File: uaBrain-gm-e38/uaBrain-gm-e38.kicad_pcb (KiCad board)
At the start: 4 copper layers, 130 x 138 mm, 3 parts, among them J1 Molex_313874018 80-pin grey, J2 Molex_313872014 73-pin black, M1 hw-uaBrain

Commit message: Upd SCH
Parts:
- added C1: 100n, hellen-one-common:C0603, F.Cu at (409.8, 70.6)
- added C10: 100n, hellen-one-common:C0603, F.Cu at (413.2, 72.6)
- added C11: 160p, hellen-one-common:C0603, F.Cu at (413.2, 74.5)
- added C12: 160p, hellen-one-common:C0603, F.Cu at (413.2, 76.5)
- added C13: 160p, hellen-one-common:C0603, F.Cu at (413.2, 78.4)
- added C14: 160p, hellen-one-common:C0603, F.Cu at (413.2, 80.4)
- added C15: 160p, hellen-one-common:C0603, F.Cu at (413.2, 82.3)
- added C16: 160p, hellen-one-common:C0603, F.Cu at (413.2, 84.3)
- added C17: 160p, hellen-one-common:C0603, F.Cu at (416.6, 70.6)
- added C18: 160p, hellen-one-common:C0603, F.Cu at (416.6, 72.6)
- added C19: 1u, hellen-one-common:C0603, F.Cu at (416.6, 74.5)
- added C2: 100n, hellen-one-common:C0603, F.Cu at (409.8, 72.6)
- added C20: 1u, hellen-one-common:C0603, F.Cu at (416.6, 76.5)
- added C21: 1u, hellen-one-common:C0603, F.Cu at (416.6, 78.4)
- added C22: 10n, Capacitor_SMD:C_0603_1608Metric, F.Cu at (410.7, 36.0)
- added C23: 10n, Capacitor_SMD:C_0603_1608Metric, F.Cu at (410.7, 38.5)
- added C24: 10n, Capacitor_SMD:C_0603_1608Metric, F.Cu at (410.7, 41.0)
- added C25: 10n, Capacitor_SMD:C_0603_1608Metric, F.Cu at (410.7, 43.6)
- added C26: 10n, Capacitor_SMD:C_0603_1608Metric, F.Cu at (410.7, 46.1)
- added C3: 100n, hellen-one-common:C0603, F.Cu at (409.8, 74.5)
- added C4: 100n, hellen-one-common:C0603, F.Cu at (409.8, 76.5)
- added C5: 100n, hellen-one-common:C0603, F.Cu at (409.8, 78.4)
- added C6: 100n, hellen-one-common:C0603, F.Cu at (409.8, 80.4)
- added C7: 100n, hellen-one-common:C0603, F.Cu at (409.8, 82.3)
- added C8: 100n, hellen-one-common:C0603, F.Cu at (409.8, 84.3)
- added C9: 100n, hellen-one-common:C0603, F.Cu at (413.2, 70.6)
- added D1: SRV05-4-P-T7, Package_TO_SOT_SMD:SOT-23-6, F.Cu at (397.4, 89.6)
- added D2: SRV05-4-P-T7, Package_TO_SOT_SMD:SOT-23-6, F.Cu at (397.4, 94.3)
- added D3: B5819W, hellen-one-common:SOD-123, F.Cu at (406.1, 36.3)
- added D4: B5819W, hellen-one-common:SOD-123, F.Cu at (406.1, 39.5)
- added D5: B5819W, hellen-one-common:SOD-123, F.Cu at (406.1, 42.6)
- added D6: B5819W, hellen-one-common:SOD-123, F.Cu at (406.1, 45.7)
- added D7: B5819W, hellen-one-common:SOD-123, F.Cu at (406.1, 48.8)
- added J3: 5569-06A2, Connector_Molex:Molex_Mini-Fit_Jr_5569-06A2_2x03_P4.20mm_Horizontal, B.Cu at (159.7, 142.7)
- added J4: 5569-06A2, Connector_Molex:Molex_Mini-Fit_Jr_5569-06A2_2x03_P4.20mm_Horizontal, B.Cu at (91.7, 142.7)
- added J5: 5569-04A2, Connector_Molex:Molex_Mini-Fit_Jr_5569-04A2_2x02_P4.20mm_Horizontal, B.Cu at (108.8, 142.7)
- added J6: 5569-16A2, Connector_Molex:Molex_Mini-Fit_Jr_5569-16A2_2x08_P4.20mm_Horizontal, B.Cu at (121.3, 142.7)
- added R1: 100, Resistor_SMD:R_2512_6332Metric_Pad1.40x3.35mm_HandSolder, F.Cu at (345.5, 60.5)
- added R10: DNP, hellen-one-common:R0603, F.Cu at (396.5, 82.4)
- added R11: 470k, hellen-one-common:R0603, F.Cu at (396.5, 84.3)
- added R12: DNP, hellen-one-common:R0603, F.Cu at (396.5, 86.3)
- added R13: 470k, hellen-one-common:R0603, F.Cu at (399.8, 70.7)
- added R14: DNP, hellen-one-common:R0603, F.Cu at (399.8, 72.6)
- added R15: 470k, hellen-one-common:R0603, F.Cu at (399.8, 74.6)
- added R16: DNP, hellen-one-common:R0603, F.Cu at (399.8, 76.5)
- added R17: 470k, hellen-one-common:R0603, F.Cu at (399.8, 78.5)
- added R18: DNP, hellen-one-common:R0603, F.Cu at (399.8, 80.4)
- added R19: 470k, hellen-one-common:R0603, F.Cu at (399.8, 82.4)
- added R2: 100, Resistor_SMD:R_2512_6332Metric_Pad1.40x3.35mm_HandSolder, F.Cu at (345.5, 65.4)
- added R20: 10k, hellen-one-common:R0603, F.Cu at (399.8, 84.3)
- added R21: 10k, hellen-one-common:R0603, F.Cu at (399.8, 86.3)
- added R22: 10k, hellen-one-common:R0603, F.Cu at (403.1, 70.7)
- added R23: 10k, hellen-one-common:R0603, F.Cu at (403.1, 72.6)
- added R24: 10k, hellen-one-common:R0603, F.Cu at (403.1, 74.6)
- added R25: 10k, hellen-one-common:R0603, F.Cu at (403.1, 76.5)
- added R26: 10k, hellen-one-common:R0603, F.Cu at (403.1, 78.5)
- added R27: 10k, hellen-one-common:R0603, F.Cu at (403.1, 80.4)
- added R28: 10k, hellen-one-common:R0603, F.Cu at (403.1, 82.4)
- added R29: 10k, hellen-one-common:R0603, F.Cu at (403.1, 84.3)
- added R3: 100, Resistor_SMD:R_2512_6332Metric_Pad1.40x3.35mm_HandSolder, F.Cu at (345.5, 70.3)
- added R30: 10k, hellen-one-common:R0603, F.Cu at (403.1, 86.3)
- added R31: 10k, hellen-one-common:R0603, F.Cu at (406.4, 70.7)
- added R32: 10k, hellen-one-common:R0603, F.Cu at (406.4, 72.6)
- added R33: 10k, hellen-one-common:R0603, F.Cu at (406.4, 74.6)
- added R34: 10k, hellen-one-common:R0603, F.Cu at (406.4, 76.5)
- added R35: 10k, hellen-one-common:R0603, F.Cu at (406.4, 78.5)
- added R36: 4.7k, hellen-one-common:R0603, F.Cu at (404.9, 51.4)
- added R37: 4.7k, hellen-one-common:R0603, F.Cu at (404.9, 53.3)
- added R38: 4.7k, hellen-one-common:R0603, F.Cu at (404.9, 55.2)
- added R39: 4.7k, hellen-one-common:R0603, F.Cu at (404.9, 57.2)
- added R4: DNP, hellen-one-common:R0603, F.Cu at (396.5, 70.7)
- added R40: 4.7k, hellen-one-common:R0603, F.Cu at (404.9, 59.1)
- added R41: 120, hellen-one-common:R0603, F.Cu at (408.2, 51.4)
- added R42: 120, hellen-one-common:R0603, F.Cu at (408.2, 53.3)
- added R43: 120, hellen-one-common:R0603, F.Cu at (408.2, 55.2)
- added R44: 120, hellen-one-common:R0603, F.Cu at (408.2, 57.2)
- added R45: 120, hellen-one-common:R0603, F.Cu at (408.2, 59.1)
- added R46: 10k, hellen-one-common:R0603, F.Cu at (411.5, 51.4)
- added R47: 10k, hellen-one-common:R0603, F.Cu at (411.5, 53.3)
- added R48: 10k, hellen-one-common:R0603, F.Cu at (411.5, 55.2)
- added R49: 10k, hellen-one-common:R0603, F.Cu at (411.5, 57.2)
- added R5: 470k, hellen-one-common:R0603, F.Cu at (396.5, 72.6)
- added R50: 10k, hellen-one-common:R0603, F.Cu at (411.5, 59.1)
- added R51: 4.7k, hellen-one-common:R0603, F.Cu at (354.3, 82.4)
- added R52: 4.7k, hellen-one-common:R0603, F.Cu at (354.3, 84.3)
- added R53: 4.7k, hellen-one-common:R0603, F.Cu at (354.3, 86.2)
- added R54: 4.7k, hellen-one-common:R0603, F.Cu at (354.3, 88.2)
- added R55: 4.7k, hellen-one-common:R0603, F.Cu at (357.6, 82.4)
- added R56: 4.7k, hellen-one-common:R0603, F.Cu at (357.6, 84.3)
- added R57: 4.7k, hellen-one-common:R0603, F.Cu at (357.6, 86.2)
- added R58: 4.7k, hellen-one-common:R0603, F.Cu at (357.6, 88.2)
- added R59: 4.7k, hellen-one-common:R0603, F.Cu at (360.9, 82.4)
- added R6: DNP, hellen-one-common:R0603, F.Cu at (396.5, 74.6)
- added R60: 4.7k, hellen-one-common:R0603, F.Cu at (360.9, 84.3)
- added R61: 4.7k, hellen-one-common:R0603, F.Cu at (360.9, 86.2)
- added R62: 4.7k, hellen-one-common:R0603, F.Cu at (360.9, 88.2)
- added R63: 4.7k, hellen-one-common:R0603, F.Cu at (351.1, 92.1)
- added R64: 4.7k, hellen-one-common:R0603, F.Cu at (351.1, 94.1)
- added R65: 4.7k, hellen-one-common:R0603, F.Cu at (351.1, 96.0)
- added R66: 4.7k, hellen-one-common:R0603, F.Cu at (351.1, 98.0)
- added R67: 4.7k, hellen-one-common:R0603, F.Cu at (354.4, 92.1)
- added R68: 4.7k, hellen-one-common:R0603, F.Cu at (354.4, 94.1)
- added R69: 4.7k, hellen-one-common:R0603, F.Cu at (354.4, 96.0)
- added R7: 470k, hellen-one-common:R0603, F.Cu at (396.5, 76.5)
- added R70: 4.7k, hellen-one-common:R0603, F.Cu at (354.4, 98.0)
- added R71: 4.7k, hellen-one-common:R0603, F.Cu at (357.7, 92.1)
- added R72: 4.7k, hellen-one-common:R0603, F.Cu at (357.7, 94.1)
- added R73: 4.7k, hellen-one-common:R0603, F.Cu at (357.7, 96.0)
- added R74: 4.7k, hellen-one-common:R0603, F.Cu at (357.7, 98.0)
- added R8: DNP, hellen-one-common:R0603, F.Cu at (396.5, 78.5)
- added R9: 470k, hellen-one-common:R0603, F.Cu at (396.5, 80.4)
- added U1: PCA9685PW, Package_SO:TSSOP-28_4.4x9.7mm_P0.65mm, F.Cu at (345.4, 78.5)
- added U10: VNLD5160TR-E, Package_SO:SOIC-8_3.9x4.9mm_P1.27mm, F.Cu at (371.0, 39.0)
- added U11: VNLD5160TR-E, Package_SO:SOIC-8_3.9x4.9mm_P1.27mm, F.Cu at (371.0, 45.6)
- added U12: VNLD5160TR-E, Package_SO:SOIC-8_3.9x4.9mm_P1.27mm, F.Cu at (371.0, 52.2)
- added U13: VNLD5160TR-E, Package_SO:SOIC-8_3.9x4.9mm_P1.27mm, F.Cu at (345.2, 94.5)
- added U14: VNLD5160TR-E, Package_SO:SOIC-8_3.9x4.9mm_P1.27mm, F.Cu at (345.2, 101.1)
- added U15: VNLD5160TR-E, Package_SO:SOIC-8_3.9x4.9mm_P1.27mm, F.Cu at (345.2, 107.7)
- added U2: MCP6004, Package_SO:TSSOP-14_4.4x5mm_P0.65mm, F.Cu at (412.4, 88.7)
- added U3: MCP6004, Package_SO:TSSOP-14_4.4x5mm_P0.65mm, F.Cu at (412.4, 95.4)
- added U4: ADS7128, Package_DFN_QFN:WQFN-16-1EP_3x3mm_P0.5mm_EP1.68x1.68mm_ThermalVias, F.Cu at (403.0, 89.9)
- added U5: BSP762TXUMA1, Package_SO:SOIC-8_3.9x4.9mm_P1.27mm, F.Cu at (399.1, 38.1)
- added U6: BSP762TXUMA1, Package_SO:SOIC-8_3.9x4.9mm_P1.27mm, F.Cu at (399.1, 44.7)
- added U7: BSP762TXUMA1, Package_SO:SOIC-8_3.9x4.9mm_P1.27mm, F.Cu at (399.1, 51.3)
- added U8: BSP762TXUMA1, Package_SO:SOIC-8_3.9x4.9mm_P1.27mm, F.Cu at (399.1, 57.9)
- added U9: BSP762TXUMA1, Package_SO:SOIC-8_3.9x4.9mm_P1.27mm, F.Cu at (399.1, 64.5)
- J1: renamed from J2; value Molex_313872014 73-pin black -> Molex_313872014_singleside
- J2: renamed from J1; value Molex_313874018 80-pin grey -> Molex_313874018_singleside
- M1: footprint kicad6-libraries:hw-uaBrain -> kicad6-libraries:hw-uaBrain-PinHeader
- moved M1 50.6 mm to (64.2, 143.6)
- moved J1 46.7 mm to (79.3, 75.9)
- moved J2 44.6 mm to (169.2, 75.8)
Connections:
- net CAN_H renamed /uaBrain-gm-e38/CAN_H
- net CAN_L renamed /uaBrain-gm-e38/CAN_L
- net IN_CAM renamed /uaBrain-gm-e38/IN_CAM
- net IN_CLT renamed /uaBrain-gm-e38/IN_CLT
- net IN_CLUTCH_SWITCH renamed /uaBrain-gm-e38/IN_CLUTCH_SWITCH
- net IN_CRANK renamed /uaBrain-gm-e38/IN_CRANK
- net IN_DIN1 renamed /uaBrain-gm-e38/IN_DIN1
- net IN_IAT renamed /uaBrain-gm-e38/IN_IAT
- net IN_KNOCK1 renamed /uaBrain-gm-e38/IN_KNOCK1
- net IN_KNOCK2 renamed /uaBrain-gm-e38/IN_KNOCK2
- net IN_MAF renamed /uaBrain-gm-e38/IN_MAF
- net IN_MAP renamed /uaBrain-gm-e38/IN_MAP
- net IN_OIL_PRESSURE renamed /uaBrain-gm-e38/IN_OIL_PRESSURE
- net IN_PPS1 renamed /uaBrain-gm-e38/IN_PPS1
- net IN_PPS2 renamed /uaBrain-gm-e38/IN_PPS2
- net IN_P/N_SWITCH renamed /uaBrain-gm-e38/IN_P/N_SWITCH
- net IN_STOP_SWITCH renamed /uaBrain-gm-e38/IN_STOP_SWITCH
- net IN_TPS1 renamed /uaBrain-gm-e38/IN_TPS1
- net IN_TPS2 renamed /uaBrain-gm-e38/IN_TPS2
- net OUT_AC_RELAY renamed /uaBrain-gm-e38/OUT_AC_RELAY
- net OUT_ETB+ renamed /uaBrain-gm-e38/OUT_ETB+
- net OUT_ETB- renamed /uaBrain-gm-e38/OUT_ETB-
- net OUT_FAN2_RELAY renamed /uaBrain-gm-e38/OUT_FAN2_RELAY
- net OUT_INJ1 renamed /uaBrain-gm-e38/OUT_INJ1
- net OUT_INJ2 renamed /uaBrain-gm-e38/OUT_INJ2
- net OUT_INJ3 renamed /uaBrain-gm-e38/OUT_INJ3
- net OUT_INJ4 renamed /uaBrain-gm-e38/OUT_INJ4
- net OUT_INJ5 renamed /uaBrain-gm-e38/OUT_INJ5
- net OUT_INJ6 renamed /uaBrain-gm-e38/OUT_INJ6
- net OUT_TACH renamed /uaBrain-gm-e38/OUT_TACH
- J1 pad 12: unconnected-(J2-Pad12) -> /uaBrain-gm-e38/IN_AC_PRESSURE
- J1 pad 16: unconnected-(J2-Pad16) -> /uaBrain-gm-e38/IN_PRIM_FUEL_LEVEL
- J1 pad 17: OUT_FAN1_RELAY -> /uaBrain-gm-e38/OUT_FAN1_RELAY
- J1 pad 20: +12V -> unconnected-(J1-Pad20)
- J1 pad 24: unconnected-(J2-Pad24) -> /uaBrain-gm-e38/IN_FTPS
- J1 pad 26: unconnected-(J2-Pad26) -> /uaBrain-gm-e38/IN_CLUTCH_POSITION
- J1 pad 47: +12V_RAW -> +12V
- J1 pad 50: unconnected-(J2-Pad50) -> /uaBrain-gm-e38/OUT_FUEL_PUMP1_RELAY_HS
- J1 pad 51: unconnected-(J2-Pad51) (its old number) -> /uaBrain-gm-e38/OUT_FUEL_PUMP2_RELAY_HS
- J1 pad 52: unconnected-(J2-Pad52) -> /uaBrain-gm-e38/OUT_STARTER_RELAY_HS
- J1 pad 57: unconnected-(J2-Pad57) -> /uaBrain-gm-e38/OUT_VSS_HS
- J1 pad 59: OUT_MAIN_RELAY -> /uaBrain-gm-e38/OUT_MAIN_RELAY
- J1 pad 61: unconnected-(J2-Pad61) -> /uaBrain-gm-e38/OUT_EVAP_VENT
- J1 pad 66: unconnected-(J2-Pad66) -> /uaBrain-gm-e38/OUT_SKIP_SHIFT_SOLENOID
- J1 pad 67: OUT_STARTER_RELAY -> /uaBrain-gm-e38/OUT_STARTER_RELAY
- J1 pad 68: OUT_CHECK_ENGINE -> /uaBrain-gm-e38/OUT_CHECK_ENGINE
- J1 pad 70: unconnected-(J2-Pad70) -> /uaBrain-gm-e38/IN_SEC_FUEL_LEVEL
- J1 pad 71: IN_VSS+ -> /uaBrain-gm-e38/IN_VSS+
- J1 pad 72: GND -> /uaBrain-gm-e38/IN_VSS-
- J1 pad 8: unconnected-(J2-Pad8) -> /uaBrain-gm-e38/IN_REVERSE_SWITCH
- J2 pad 10: unconnected-(J1-Pad10) (its old number) -> /uaBrain-gm-e38/OUT_DOD_CYL1
- J2 pad 11: unconnected-(J1-Pad11) (its old number) -> /uaBrain-gm-e38/OUT_DOD_CYL2
- J2 pad 12: OUT_BK1S1HTR -> unconnected-(J2-Pad12)
- J2 pad 13: OUT_BK2S1HTR -> unconnected-(J2-Pad13)
- J2 pad 14: unconnected-(J1-Pad14) (its old number) -> /uaBrain-gm-e38/OUT_DOD_CYL4
- J2 pad 16: unconnected-(J1-Pad16) -> /uaBrain-gm-e38/OUT_VVT_HS
- J2 pad 17: unconnected-(J1-Pad17) -> /uaBrain-gm-e38/OUT_INJ8
- J2 pad 23: unconnected-(J1-Pad23) -> /uaBrain-gm-e38/IN_ATF_TEMP
- J2 pad 33: unconnected-(J1-Pad33) -> /uaBrain-gm-e38/IN_OIL_LEVEL_SWITCH
- J2 pad 40: unconnected-(J1-Pad40) -> /uaBrain-gm-e38/OUT_INJ7
- J2 pad 57: unconnected-(J1-Pad57) -> /uaBrain-gm-e38/IN_BK1S1SIG
- J2 pad 61: unconnected-(J1-Pad61) -> /uaBrain-gm-e38/OUT_ALT_LIGHT
- J2 pad 70: OUT_IGN1 -> /uaBrain-gm-e38/OUT_IGN1_6
- J2 pad 71: unconnected-(J1-Pad71) -> /uaBrain-gm-e38/OUT_IGN8_5
- J2 pad 72: unconnected-(J1-Pad72) -> /uaBrain-gm-e38/OUT_IGN7_4
- J2 pad 73: OUT_IGN2 -> /uaBrain-gm-e38/OUT_IGN2_3
- J2 pad 74: OUT_IGN6 -> /uaBrain-gm-e38/OUT_IGN1_6
- J2 pad 75: OUT_IGN5 -> /uaBrain-gm-e38/OUT_IGN8_5
- J2 pad 76: OUT_IGN4 -> /uaBrain-gm-e38/OUT_IGN7_4
- J2 pad 77: OUT_IGN3 -> /uaBrain-gm-e38/OUT_IGN2_3
- J2 pad 8: OUT_EVAP_PURGE -> unconnected-(J2-Pad8)
- J2 pad 9: unconnected-(J1-Pad9) -> /uaBrain-gm-e38/OUT_DOD_CYL3
- M1 pad A1: unconnected-(M1A-6_WBO1_Un-PadA1) -> /uaBrain-gm-e38/6_WBO1_Un
- M1 pad A2: unconnected-(M1A-5_WBO1_Rtrim-PadA2) -> /uaBrain-gm-e38/5_WBO1_Rtrim
- M1 pad A3: unconnected-(M1A-1_WBO1_Ip-PadA3)_1 -> /uaBrain-gm-e38/1_WBO1_Ip
- M1 pad A4: unconnected-(M1A-2_WBO1_Vm-PadA4)_1 -> /uaBrain-gm-e38/2_WBO1_Vm
- M1 pad A5: unconnected-(M1A-3_WBO1_Heater-PadA5) -> /uaBrain-gm-e38/3_WBO1_Heater
- M1 pad A7: unconnected-(M1A-EGT1--PadA7)_1 -> /uaBrain-gm-e38/EGT1-
- M1 pad A8: unconnected-(M1A-EGT1+-PadA8)_1 -> /uaBrain-gm-e38/EGT1+
- M1 pad B1: OUT_IGN1 -> /uaBrain-gm-e38/OUT_IGN1_6
- M1 pad B2: OUT_IGN2 -> /uaBrain-gm-e38/OUT_IGN8_5
- M1 pad B3: OUT_IGN3 -> /uaBrain-gm-e38/OUT_IGN7_4
- M1 pad C1: unconnected-(M1A-VR_DISCRETE--PadC1)_1 -> /uaBrain-gm-e38/IN_VSS-
- M1 pad C2: unconnected-(M1A-VR_DISCRETE+-PadC2) -> /uaBrain-gm-e38/IN_VSS+
- M1 pad D5: unconnected-(M1A-+3.3VA-PadD5)_1 -> +3.3VA
- M1 pad D6: unconnected-(M1A-+3.3V-PadD6)_1 -> +3.3V
- M1 pad D7: unconnected-(M1A-+5VA-PadD7)_1 -> +5VA
- M1 pad D8: unconnected-(M1A-+5V-PadD8) -> +5V
- M1 pad F1: unconnected-(M1B-OUT_DC2--PadF1)_1 -> /uaBrain-gm-e38/OUT_DC2-
- M1 pad F2: unconnected-(M1B-OUT_DC2+-PadF2)_1 -> /uaBrain-gm-e38/OUT_DC2+
- M1 pad G4: unconnected-(M1B-CAN2+-PadG4) -> /uaBrain-gm-e38/CAN2+
- M1 pad G5: unconnected-(M1B-CAN2--PadG5)_1 -> /uaBrain-gm-e38/CAN2-
- M1 pad G6: OUT_EVAP_PURGE -> /uaBrain-gm-e38/OUT_SKIP_SHIFT_SOLENOID
- M1 pad G7: OUT_STARTER_RELAY -> /uaBrain-gm-e38/OUT_DOD_CYL1
- M1 pad H1: unconnected-(M1B-6_WBO2_Un-PadH1)_1 -> /uaBrain-gm-e38/6_WBO2_Un
- M1 pad H2: unconnected-(M1B-5_WBO2_Rtrim-PadH2) -> /uaBrain-gm-e38/5_WBO2_Rtrim
- M1 pad H3: unconnected-(M1B-1_WBO2_Ip-PadH3) -> /uaBrain-gm-e38/1_WBO2_Ip
- M1 pad H4: unconnected-(M1B-2_WBO2_Vm-PadH4) -> /uaBrain-gm-e38/2_WBO2_Vm
- M1 pad H5: unconnected-(M1B-3_WBO2_Heater-PadH5)_1 -> /uaBrain-gm-e38/3_WBO2_Heater
- M1 pad H7: unconnected-(M1B-EGT2--PadH7) -> /uaBrain-gm-e38/EGT2-
- M1 pad H8: unconnected-(M1B-EGT2+-PadH8) -> /uaBrain-gm-e38/EGT2+
- M1 pad J1: OUT_IGN4 -> /uaBrain-gm-e38/OUT_IGN2_3
- M1 pad J2: OUT_IGN5 -> /uaBrain-gm-e38/ALT_LIGHT
- M1 pad J3: OUT_IGN6 -> /uaBrain-gm-e38/MAIN_RELAY
- M1 pad K1: unconnected-(M1B-VR_MAX9924--PadK1) -> /uaBrain-gm-e38/VR_MAX9924-
- M1 pad K2: unconnected-(M1B-VR_MAX9924+-PadK2) -> /uaBrain-gm-e38/VR_MAX9924+
- M1 pad K4: IN_VSS+ -> /uaBrain-gm-e38/IN_REVERSE_SWITCH
- M1 pad K7: OUT_CHECK_ENGINE -> /uaBrain-gm-e38/OUT_DOD_CYL2
- M1 pad L5: unconnected-(M1C-+3.3VA-PadL5) -> +3.3VA
- M1 pad L6: /SDA -> /uaBrain-gm-e38/SDA
- M1 pad L7: unconnected-(M1C-+5VA-PadL7) -> +5VA
- M1 pad L8: /SCL -> /uaBrain-gm-e38/SCL
- M1 pad M5: OUT_BK1S1HTR -> /uaBrain-gm-e38/OUT_INJ7
- M1 pad M6: OUT_BK2S1HTR -> /uaBrain-gm-e38/OUT_INJ8
- M1 pad M7: OUT_MAIN_RELAY -> /uaBrain-gm-e38/OUT_DOD_CYL3
- M1 pad M8: OUT_FAN1_RELAY -> /uaBrain-gm-e38/OUT_DOD_CYL4
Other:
- board size 130 x 138 mm -> 149 x 105.9 mm

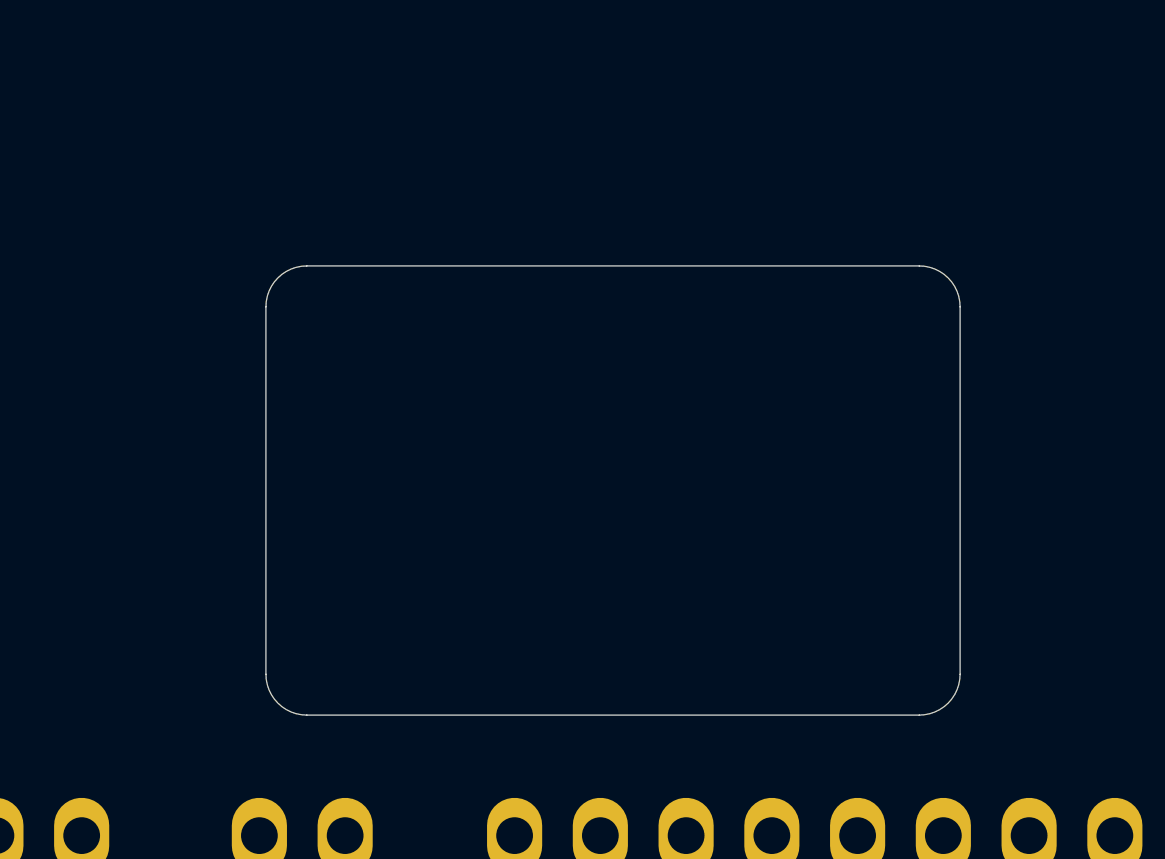
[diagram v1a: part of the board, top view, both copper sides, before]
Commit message: Upd SCH
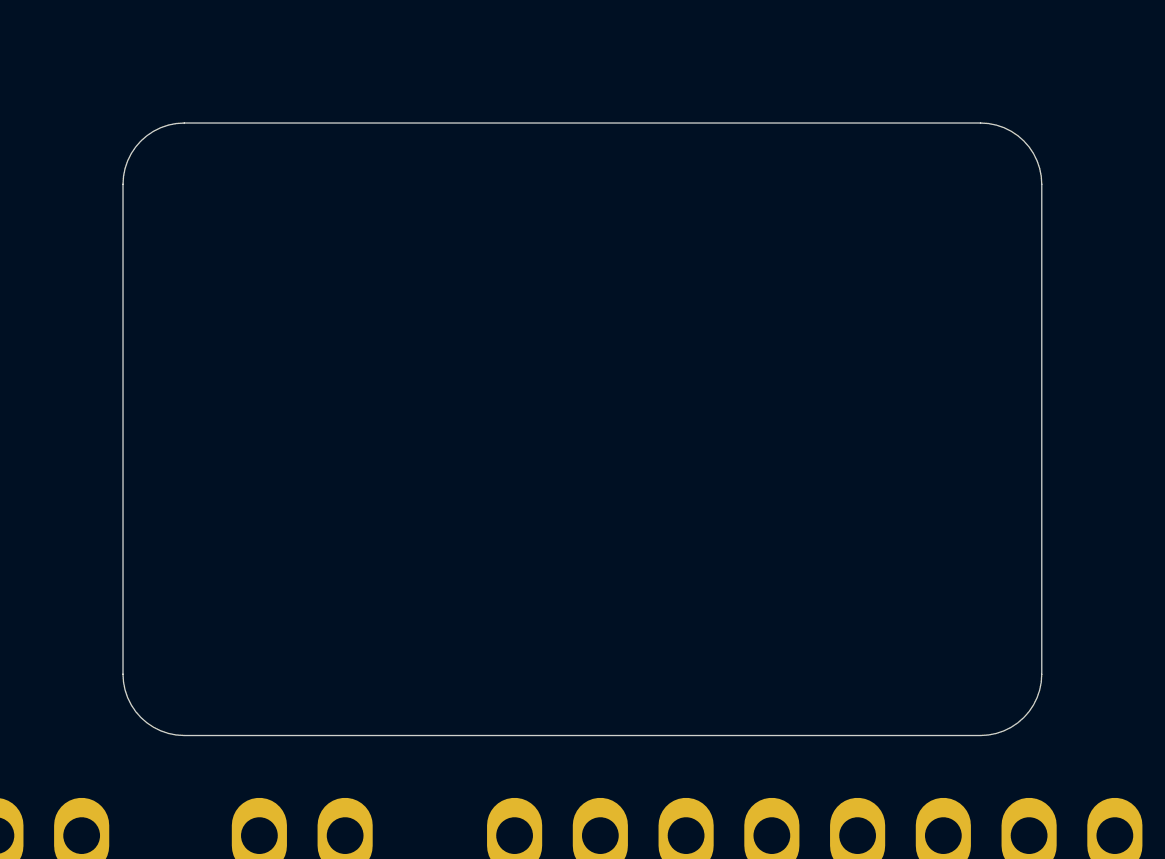
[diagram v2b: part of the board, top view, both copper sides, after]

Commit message: uaBrain-e38 rev a
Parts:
- removed R51, R52, R53, R54, R55, R56, R57, R58, R59, R60, R61, R62: 4.7k, hellen-one-common:R0603
- removed U10, U11, U12: VNLD5160TR-E, Package_SO:SOIC-8_3.9x4.9mm_P1.27mm
- added C27: 1u, hellen-one-common:C0603, B.Cu at (142.0, 70.9)
- added G1: RUSEFI_LOGO, kicad6-libraries:rusefi_logo, B.Cu at (153.0, 66.0)
- added H1: M3, MountingHole:MountingHole_3.2mm_M3_Pad_Via, F.Cu at (200.1, 56.0)
- added H2: M3, MountingHole:MountingHole_3.2mm_M3_Pad_Via, F.Cu at (59.1, 56.0)
- added H3: M3, MountingHole:MountingHole_3.2mm_M3_Pad_Via, F.Cu at (59.1, 152.0)
- added H4: M3, MountingHole:MountingHole_3.2mm_M3_Pad_Via, F.Cu at (200.1, 152.0)
- added J10: PH2.54-01-16PZD, Connector_PinHeader_2.54mm:PinHeader_1x16_P2.54mm_Vertical, F.Cu at (170.6, 61.2)
- added J11: PH2.54-01-16PZD, Connector_PinHeader_2.54mm:PinHeader_1x16_P2.54mm_Vertical, F.Cu at (130.0, 61.2)
- added J12: PH2.54-01-16PZD, Connector_PinHeader_2.54mm:PinHeader_1x16_P2.54mm_Vertical, F.Cu at (89.3, 61.2)
- added J13: PH2.54-01-16PZD, Connector_PinHeader_2.54mm:PinHeader_1x16_P2.54mm_Vertical, F.Cu at (67.7, 82.4)
- added J14: PH2.54-01-16PZD, Connector_PinHeader_2.54mm:PinHeader_1x16_P2.54mm_Vertical, F.Cu at (67.7, 123.0)
- added J7: C4201WR-F-2x8P, Connector_Molex:Molex_Mini-Fit_Jr_5569-16A2_2x08_P4.20mm_Horizontal, B.Cu at (103.3, 142.7)
- added J8: PH2.54-01-16PZD, Connector_PinHeader_2.54mm:PinHeader_1x16_P2.54mm_Vertical, F.Cu at (192.2, 123.0)
- added J9: PH2.54-01-16PZD, Connector_PinHeader_2.54mm:PinHeader_1x16_P2.54mm_Vertical, F.Cu at (192.2, 82.4)
- C11, C12, C13, C14, C15, C16, C17, C18, C20, C21, D1, D2, R10, R12, R16, R20, R21, R22, R23, R24, R25, R26, R27, R28, R29, R30, R31, R32, R33, R34, R35, R6, R8, U1, U13, U14, U15, U2, U3, U4, U5, U6, U7, U8, U9: moved to B.Cu
- J6: value 5569-16A2 -> C4201WR-F-2x8P
- R11, R13, R17, R7, R9: value 470k -> 680k
- R14: value DNP -> 10k; moved to B.Cu
- R15, R19, R5: value 470k -> DNP
- R18, R4: value DNP -> 4.7k; moved to B.Cu
- moved C25 310.7 mm to (103.3, 88.9)
- moved R49 305.4 mm to (107.5, 85.1), turned to 180 degrees
- moved D6 305.3 mm to (103.6, 86.8)
- moved R39 302.9 mm to (103.3, 84.8), turned to 180 degrees
- moved R44 302.4 mm to (107.5, 88.9), turned to 180 degrees
- moved C22 300.2 mm to (115.0, 87.7)
- moved C23 298.8 mm to (115.0, 81.1)
- moved C24 297.6 mm to (115.0, 74.5)
- moved U8 295.5 mm to (105.0, 87.0)
- moved D3 294.9 mm to (115.3, 85.6)
- moved R46 294.2 mm to (119.2, 83.8), turned to 180 degrees
- moved D4 293.4 mm to (115.3, 79.0)
- moved R47 293.4 mm to (119.2, 77.3), turned to 180 degrees
- moved R48 292.8 mm to (119.2, 70.7), turned to 180 degrees
- moved D5 292.3 mm to (115.3, 72.4)
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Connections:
- net /uaBrain-gm-e38/1_WBO1_Ip renamed /1_WBO1_Ip
- net /uaBrain-gm-e38/1_WBO2_Ip renamed /1_WBO2_Ip
- net /uaBrain-gm-e38/2_WBO1_Vm renamed /2_WBO1_Vm
- net /uaBrain-gm-e38/2_WBO2_Vm renamed /2_WBO2_Vm
- net /uaBrain-gm-e38/3_WBO1_Heater renamed /3_WBO1_Heater
- net /uaBrain-gm-e38/3_WBO2_Heater renamed /3_WBO2_Heater
- net /uaBrain-gm-e38/5_WBO1_Rtrim renamed /5_WBO1_Rtrim
- net /uaBrain-gm-e38/5_WBO2_Rtrim renamed /5_WBO2_Rtrim
- net /uaBrain-gm-e38/6_WBO1_Un renamed /6_WBO1_Un
- net /uaBrain-gm-e38/6_WBO2_Un renamed /6_WBO2_Un
- net /uaBrain-gm-e38/CAN2+ renamed /CAN2+
- net /uaBrain-gm-e38/CAN2- renamed /CAN2-
- net /uaBrain-gm-e38/CAN_H renamed /CAN_H
- net /uaBrain-gm-e38/CAN_L renamed /CAN_L
- net /uaBrain-gm-e38/EGT1+ renamed /EGT1+
- net /uaBrain-gm-e38/EGT1- renamed /EGT1-
- net /uaBrain-gm-e38/EGT2+ renamed /EGT2+
- net /uaBrain-gm-e38/EGT2- renamed /EGT2-
- net /uaBrain-gm-e38/HS5/IN1 renamed /HS5/IN1
- net /uaBrain-gm-e38/HS5/IN2 renamed /HS5/IN2
- net /uaBrain-gm-e38/HS5/IN3 renamed /HS5/IN3
- net /uaBrain-gm-e38/HS5/IN4 renamed /HS5/IN4
- net /uaBrain-gm-e38/HS5/IN5 renamed /HS5/IN5
- net /uaBrain-gm-e38/IN_CAM renamed /IN_CAM
- net /uaBrain-gm-e38/IN_CLT renamed /IN_CLT
- net /uaBrain-gm-e38/IN_CLUTCH_SWITCH renamed /IN_CLUTCH_SWITCH
- net /uaBrain-gm-e38/IN_CRANK renamed /IN_CRANK
- net /uaBrain-gm-e38/IN_DIN1 renamed /IN_FLEX
- net /uaBrain-gm-e38/IN_IAT renamed /IN_IAT
- net /uaBrain-gm-e38/IN_KNOCK1 renamed /IN_KNOCK1
- net /uaBrain-gm-e38/IN_KNOCK2 renamed /IN_KNOCK2
- net /uaBrain-gm-e38/IN_MAF renamed /IN_MAF
- net /uaBrain-gm-e38/IN_MAP renamed /IN_MAP
- net /uaBrain-gm-e38/IN_OIL_PRESSURE renamed /IN_OIL_PRESSURE
- net /uaBrain-gm-e38/IN_PPS1 renamed /IN_PPS1
- net /uaBrain-gm-e38/IN_PPS2 renamed /IN_PPS2
- net /uaBrain-gm-e38/IN_P/N_SWITCH renamed /IN_P/N_SWITCH
- net /uaBrain-gm-e38/IN_REVERSE_SWITCH renamed /IN_REVERSE_SWITCH
- net /uaBrain-gm-e38/IN_STOP_SWITCH renamed /IN_STOP_SWITCH
- net /uaBrain-gm-e38/IN_TPS1 renamed /IN_TPS1
- net /uaBrain-gm-e38/IN_TPS2 renamed /IN_TPS2
- net /uaBrain-gm-e38/IN_VSS+ renamed /IN_VSS+
- net /uaBrain-gm-e38/IN_VSS- renamed /IN_VSS-
- net /uaBrain-gm-e38/OUT_AC_RELAY renamed /OUT_AC_RELAY
- net /uaBrain-gm-e38/OUT_DC2+ renamed /OUT_DC2+
- net /uaBrain-gm-e38/OUT_DC2- renamed /OUT_DC2-
- net /uaBrain-gm-e38/OUT_DOD_CYL1 renamed /OUT_DOD_CYL1
- net /uaBrain-gm-e38/OUT_DOD_CYL2 renamed /OUT_DOD_CYL2
- net /uaBrain-gm-e38/OUT_DOD_CYL3 renamed /OUT_DOD_CYL3
- net /uaBrain-gm-e38/OUT_DOD_CYL4 renamed /OUT_DOD_CYL4
- net /uaBrain-gm-e38/OUT_ETB+ renamed /OUT_ETB+
- net /uaBrain-gm-e38/OUT_ETB- renamed /OUT_ETB-
- net /uaBrain-gm-e38/OUT_FAN2_RELAY renamed /OUT_FAN2_RELAY
- net /uaBrain-gm-e38/OUT_FUEL_PUMP1_RELAY_HS renamed /OUT_FUEL_PUMP1_RELAY_HS
- net /uaBrain-gm-e38/OUT_FUEL_PUMP2_RELAY_HS renamed /OUT_FUEL_PUMP2_RELAY_HS
- net /uaBrain-gm-e38/OUT_IGN1_6 renamed /OUT_IGN1_6
- net /uaBrain-gm-e38/OUT_IGN2_3 renamed /OUT_IGN2_3
- net /uaBrain-gm-e38/OUT_IGN7_4 renamed /OUT_IGN7_4
- net /uaBrain-gm-e38/OUT_IGN8_5 renamed /OUT_IGN8_5
- net /uaBrain-gm-e38/OUT_INJ1 renamed /OUT_INJ1
- net /uaBrain-gm-e38/OUT_INJ2 renamed /OUT_INJ2
- net /uaBrain-gm-e38/OUT_INJ3 renamed /OUT_INJ3
- net /uaBrain-gm-e38/OUT_INJ4 renamed /OUT_INJ4
- net /uaBrain-gm-e38/OUT_INJ5 renamed /OUT_INJ5
- net /uaBrain-gm-e38/OUT_INJ6 renamed /OUT_INJ6
- net /uaBrain-gm-e38/OUT_INJ7 renamed /OUT_INJ7
- net /uaBrain-gm-e38/OUT_INJ8 renamed /OUT_INJ8
- net /uaBrain-gm-e38/OUT_SKIP_SHIFT_SOLENOID renamed /OUT_SKIP_SHIFT_SOLENOID
- net /uaBrain-gm-e38/OUT_STARTER_RELAY_HS renamed /OUT_STARTER_RELAY_HS
- net /uaBrain-gm-e38/OUT_TACH renamed /OUT_TACH
- net /uaBrain-gm-e38/OUT_VSS_HS renamed /OUT_VSS_HS
- net /uaBrain-gm-e38/OUT_VVT_HS renamed /OUT_VVT_HS
- net /uaBrain-gm-e38/SCL renamed /SCL
- net /uaBrain-gm-e38/SDA renamed /SDA
- net /uaBrain-gm-e38/VR_MAX9924+ renamed /VR_MAX9924+
- net /uaBrain-gm-e38/VR_MAX9924- renamed /VR_MAX9924-
- C1 pad 1: GND -> GNDA
- C10 pad 1: GND -> GNDA
- C11 pad 1: GND -> GNDA
- C11 pad 2: /uaBrain-gm-e38/IN_ATF_TEMP -> /I2C ADC inputs/ADC0
- C12 pad 1: GND -> GNDA
- C12 pad 2: /uaBrain-gm-e38/IN_PRIM_FUEL_LEVEL -> /I2C ADC inputs/ADC4
- C13 pad 1: GND -> GNDA
- C13 pad 2: /uaBrain-gm-e38/IN_AC_PRESSURE -> /I2C ADC inputs/ADC1
- C14 pad 1: GND -> GNDA
- C14 pad 2: /uaBrain-gm-e38/IN_SEC_FUEL_LEVEL -> /I2C ADC inputs/ADC5
- C15 pad 1: GND -> GNDA
- C15 pad 2: /uaBrain-gm-e38/IN_FTPS -> /I2C ADC inputs/ADC2
- C16 pad 1: GND -> GNDA
- C16 pad 2: /uaBrain-gm-e38/IN_OIL_LEVEL_SWITCH -> /I2C ADC inputs/ADC6
- C17 pad 1: GND -> GNDA
- C17 pad 2: /uaBrain-gm-e38/IN_CLUTCH_POSITION -> /I2C ADC inputs/ADC3
- C18 pad 1: GND -> GNDA
- C18 pad 2: /uaBrain-gm-e38/IN_BK1S1SIG -> /I2C ADC inputs/ADC7
- C19 pad 1: GND -> GNDA
- C2 pad 1: GND -> GNDA
- C20 pad 1: GND -> GNDA
- C21 pad 1: GND -> GNDA
- C3 pad 1: GND -> GNDA
- C4 pad 1: GND -> GNDA
- C5 pad 1: GND -> GNDA
- C6 pad 1: GND -> GNDA
- C7 pad 1: GND -> GNDA
- C8 pad 1: GND -> GNDA
- C9 pad 1: GND -> GNDA
- D1 pad 2: GND -> GNDA
- D2 pad 2: GND -> GNDA
- J1 pad 12: /uaBrain-gm-e38/IN_AC_PRESSURE -> /IN_AC_PRESSURE
- J1 pad 16: /uaBrain-gm-e38/IN_PRIM_FUEL_LEVEL -> /IN_PRIM_FUEL_LEVEL
- J1 pad 17: /uaBrain-gm-e38/OUT_FAN1_RELAY -> /OUT_FAN1_RELAY
- J1 pad 24: /uaBrain-gm-e38/IN_FTPS -> /IN_FUEL_TANK_PRESSURE
- J1 pad 26: /uaBrain-gm-e38/IN_CLUTCH_POSITION -> /IN_CLUTCH_POSITION
- J1 pad 59: /uaBrain-gm-e38/OUT_MAIN_RELAY -> /OUT_MAIN_RELAY
- J1 pad 61: /uaBrain-gm-e38/OUT_EVAP_VENT -> /OUT_EVAP_VENT
- J1 pad 67: /uaBrain-gm-e38/OUT_STARTER_RELAY -> /OUT_STARTER_RELAY
- J1 pad 68: /uaBrain-gm-e38/OUT_CHECK_ENGINE -> /OUT_CHECK_ENGINE
- J1 pad 70: /uaBrain-gm-e38/IN_SEC_FUEL_LEVEL -> /IN_SEC_FUEL_LEVEL
- J2 pad 23: /uaBrain-gm-e38/IN_ATF_TEMP -> /IN_ATF_TEMP
- J2 pad 33: /uaBrain-gm-e38/IN_OIL_LEVEL_SWITCH -> /IN_OIL_LEVEL_SWITCH
- J2 pad 57: /uaBrain-gm-e38/IN_BK1S1SIG -> /IN_BK1S1SIG
- J2 pad 61: /uaBrain-gm-e38/OUT_ALT_LIGHT -> /OUT_ALT_LIGHT
- J6 pad 8: /uaBrain-gm-e38/IN_BK1S1SIG -> /IN_BK1S1SIG
- M1 pad J2: /uaBrain-gm-e38/ALT_LIGHT -> /ALT_LIGHT
- M1 pad J3: /uaBrain-gm-e38/MAIN_RELAY -> /MAIN_RELAY
- R1 pad 2: /uaBrain-gm-e38/IN_PRIM_FUEL_LEVEL -> /IN_PRIM_FUEL_LEVEL
- R10 pad 1: /uaBrain-gm-e38/IN_SEC_FUEL_LEVEL -> /IN_SEC_FUEL_LEVEL
- R11 pad 1: GND -> GNDA
- R11 pad 2: /uaBrain-gm-e38/IN_SEC_FUEL_LEVEL -> /IN_SEC_FUEL_LEVEL
- R12 pad 1: /uaBrain-gm-e38/IN_FTPS -> /IN_FUEL_TANK_PRESSURE
- R13 pad 1: GND -> GNDA
- R13 pad 2: /uaBrain-gm-e38/IN_FTPS -> /IN_FUEL_TANK_PRESSURE
- R14 pad 1: /uaBrain-gm-e38/IN_OIL_LEVEL_SWITCH -> /IN_OIL_LEVEL_SWITCH
- R15 pad 1: GND -> GNDA
- R15 pad 2: /uaBrain-gm-e38/IN_OIL_LEVEL_SWITCH -> /IN_OIL_LEVEL_SWITCH
- R16 pad 1: /uaBrain-gm-e38/IN_CLUTCH_POSITION -> /IN_CLUTCH_POSITION
- R17 pad 1: GND -> GNDA
- R17 pad 2: /uaBrain-gm-e38/IN_CLUTCH_POSITION -> /IN_CLUTCH_POSITION
- R18 pad 1: /uaBrain-gm-e38/IN_BK1S1SIG -> /IN_BK1S1SIG
- R19 pad 1: GND -> GNDA
- R19 pad 2: /uaBrain-gm-e38/IN_BK1S1SIG -> /IN_BK1S1SIG
- R2 pad 2: /uaBrain-gm-e38/IN_SEC_FUEL_LEVEL -> /IN_SEC_FUEL_LEVEL
- R20 pad 2: /uaBrain-gm-e38/IN_ATF_TEMP -> /IN_ATF_TEMP
- R21 pad 2: /uaBrain-gm-e38/IN_AC_PRESSURE -> /IN_AC_PRESSURE
- R22 pad 2: /uaBrain-gm-e38/IN_FTPS -> /IN_FUEL_TANK_PRESSURE
- R23 pad 2: /uaBrain-gm-e38/IN_CLUTCH_POSITION -> /IN_CLUTCH_POSITION
- R24 pad 2: /uaBrain-gm-e38/IN_PRIM_FUEL_LEVEL -> /IN_PRIM_FUEL_LEVEL
- R25 pad 2: /uaBrain-gm-e38/IN_SEC_FUEL_LEVEL -> /IN_SEC_FUEL_LEVEL
- R26 pad 2: /uaBrain-gm-e38/IN_OIL_LEVEL_SWITCH -> /IN_OIL_LEVEL_SWITCH
- R27 pad 2: /uaBrain-gm-e38/IN_BK1S1SIG -> /IN_BK1S1SIG
- R28 pad 1: /uaBrain-gm-e38/IN_ATF_TEMP -> /I2C ADC inputs/ADC0
- R29 pad 1: /uaBrain-gm-e38/IN_AC_PRESSURE -> /I2C ADC inputs/ADC1
- R3 pad 2: /uaBrain-gm-e38/OUT_ALT_LIGHT -> /OUT_ALT_LIGHT
- R30 pad 1: /uaBrain-gm-e38/IN_FTPS -> /I2C ADC inputs/ADC2
- R31 pad 1: /uaBrain-gm-e38/IN_CLUTCH_POSITION -> /I2C ADC inputs/ADC3
- R32 pad 1: /uaBrain-gm-e38/IN_PRIM_FUEL_LEVEL -> /I2C ADC inputs/ADC4
- R33 pad 1: /uaBrain-gm-e38/IN_SEC_FUEL_LEVEL -> /I2C ADC inputs/ADC5
- R34 pad 1: /uaBrain-gm-e38/IN_OIL_LEVEL_SWITCH -> /I2C ADC inputs/ADC6
- R35 pad 1: /uaBrain-gm-e38/IN_BK1S1SIG -> /I2C ADC inputs/ADC7
- R4 pad 1: /uaBrain-gm-e38/IN_ATF_TEMP -> /IN_ATF_TEMP
- R5 pad 1: GND -> GNDA
- R5 pad 2: /uaBrain-gm-e38/IN_ATF_TEMP -> /IN_ATF_TEMP
- R6 pad 1: /uaBrain-gm-e38/IN_PRIM_FUEL_LEVEL -> /IN_PRIM_FUEL_LEVEL
- R63 pad 1: Net-(R63-Pad1) -> /ALT_LIGHT
- R64 pad 1: Net-(R64-Pad1) -> /MAIN_RELAY
- R65 pad 1: Net-(R65-Pad1) -> /STARTER_RELAY
- R66 pad 1: Net-(R66-Pad1) -> /CHECK_ENGINE
- R67 pad 1: Net-(R67-Pad1) -> /EVAP_VENT
- R68 pad 1: Net-(R68-Pad1) -> /FAN1_RELAY
- R69 pad 2: Net-(R63-Pad1) -> /ALT_LIGHT
- R7 pad 1: GND -> GNDA
- R7 pad 2: /uaBrain-gm-e38/IN_PRIM_FUEL_LEVEL -> /IN_PRIM_FUEL_LEVEL
- R70 pad 2: Net-(R64-Pad1) -> /MAIN_RELAY
- R71 pad 2: Net-(R65-Pad1) -> /STARTER_RELAY
- R72 pad 2: Net-(R66-Pad1) -> /CHECK_ENGINE
- R73 pad 2: Net-(R67-Pad1) -> /EVAP_VENT
- R74 pad 2: Net-(R68-Pad1) -> /FAN1_RELAY
- R8 pad 1: /uaBrain-gm-e38/IN_AC_PRESSURE -> /IN_AC_PRESSURE
- R9 pad 1: GND -> GNDA
- R9 pad 2: /uaBrain-gm-e38/IN_AC_PRESSURE -> /IN_AC_PRESSURE
- U1 pad 11: /uaBrain-gm-e38/STARTER_RELAY -> /STARTER_RELAY
- U1 pad 12: /uaBrain-gm-e38/CHECK_ENGINE -> /CHECK_ENGINE
- U1 pad 13: /uaBrain-gm-e38/EVAP_VENT -> /EVAP_VENT
- U1 pad 15: /uaBrain-gm-e38/FAN1_RELAY -> /FAN1_RELAY
- U13 pad 6: unconnected-(U13-D2-Pad6) -> /OUT_MAIN_RELAY
- U13 pad 8: unconnected-(U13-D1-Pad8) -> /OUT_ALT_LIGHT
- U14 pad 6: unconnected-(U14-D2-Pad6) -> /OUT_CHECK_ENGINE
- U14 pad 8: unconnected-(U14-D1-Pad8) -> /OUT_STARTER_RELAY
- U15 pad 6: unconnected-(U15-D2-Pad6) -> /OUT_FAN1_RELAY
- U15 pad 8: unconnected-(U15-D1-Pad8) -> /OUT_EVAP_VENT
- U2 pad 11: GND -> GNDA
- U3 pad 11: GND -> GNDA
- U4 pad 1: /uaBrain-gm-e38/IN_FTPS -> /I2C ADC inputs/ADC2
- U4 pad 15: /uaBrain-gm-e38/IN_ATF_TEMP -> /I2C ADC inputs/ADC0
- U4 pad 16: /uaBrain-gm-e38/IN_AC_PRESSURE -> /I2C ADC inputs/ADC1
- U4 pad 17: GND -> GNDA
- U4 pad 2: /uaBrain-gm-e38/IN_CLUTCH_POSITION -> /I2C ADC inputs/ADC3
- U4 pad 3: /uaBrain-gm-e38/IN_PRIM_FUEL_LEVEL -> /I2C ADC inputs/ADC4
- U4 pad 4: /uaBrain-gm-e38/IN_SEC_FUEL_LEVEL -> /I2C ADC inputs/ADC5
- U4 pad 5: /uaBrain-gm-e38/IN_OIL_LEVEL_SWITCH -> /I2C ADC inputs/ADC6
- U4 pad 6: /uaBrain-gm-e38/IN_BK1S1SIG -> /I2C ADC inputs/ADC7
- U4 pad 9: GND -> GNDA
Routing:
- net GNDA: track 0.00 -> 783.3 mm, vias 0 -> 37
- net +5VP: track 0.00 -> 402.6 mm, vias 0 -> 14
- net /1_WBO2_Ip: track 0.00 -> 342.0 mm, vias 0 -> 4
- net +12V_RAW: track 0.00 -> 308.5 mm, vias 0 -> 10
- net /OUT_DOD_CYL2: track 0.00 -> 274.0 mm, vias 0 -> 8
- net +5VA: track 0.00 -> 257.7 mm, vias 0 -> 23
- net +3.3VA: track 0.00 -> 211.4 mm, vias 0 -> 7
- net /OUT_INJ8: track 0.00 -> 205.9 mm, vias 0 -> 4
- net /IN_MAF: track 0.00 -> 204.1 mm, vias 0 -> 6
- net /OUT_INJ7: track 0.00 -> 191.1 mm, vias 0 -> 1
- net /OUT_DOD_CYL3: track 0.00 -> 189.5 mm, vias 0 -> 3
- net /5_WBO2_Rtrim: track 0.00 -> 185.2 mm, vias 0 -> 4
- net /3_WBO2_Heater: track 0.00 -> 173.3 mm
- net /VR_MAX9924-: track 0.00 -> 170.3 mm, vias 0 -> 4
- net /OUT_DOD_CYL4: track 0.00 -> 170.1 mm, vias 0 -> 2
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- added copper zone on B.Cu, net GND
- added copper zone on F.Cu, net GND
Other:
- board size 149 x 105.9 mm -> 149 x 104 mm
- copper layers 4 -> 2
- board text added: "Always looking for C/C++/PHP/Java developers"
- board text added: "https://rusefi.com/s/mission"
- board text added: "rusefi.com/s/uabrain-e38"
- board text added: "uaBrain-gm-e38 rev. a"
